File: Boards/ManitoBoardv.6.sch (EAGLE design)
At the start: 46 parts, among them U1 BLUETOOTH-RN41", U2 ATMEGA328P

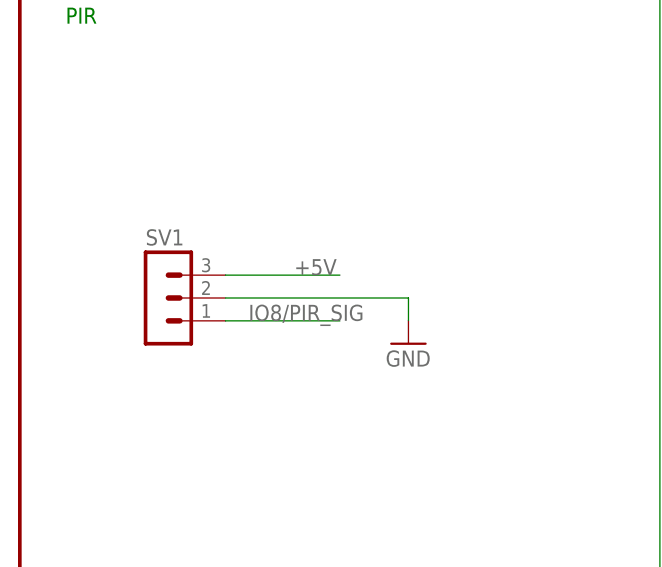
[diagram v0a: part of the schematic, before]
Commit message: Board with Layout
First complete layout now version .6
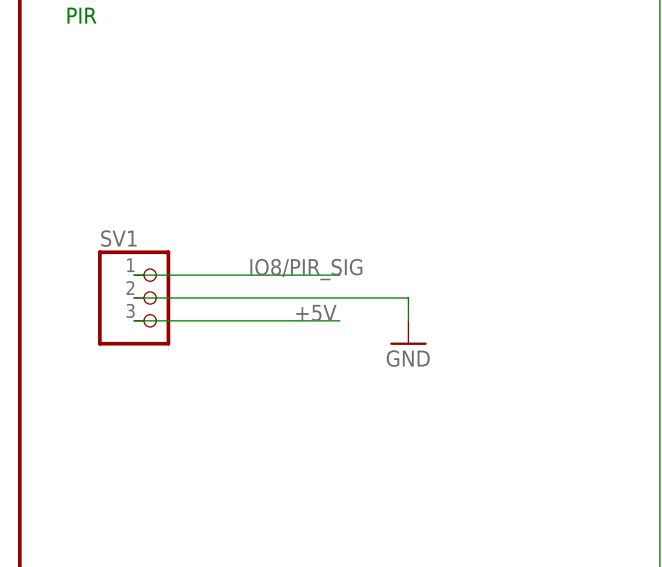
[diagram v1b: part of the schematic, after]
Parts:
- SV1: device con-lstb:MA03-1 -> adafruit:PINHD-1X3
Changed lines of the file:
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@@
 <part name="P+11" library="SparkFun" deviceset="VCC" device="" value="3.3V"/>
 <part name="P+4" library="supply1" deviceset="+5V" device=""/>
-<part name="SV1" library="con-lstb" deviceset="MA03-1" device=""/>
+<part name="SV1" library="adafruit" deviceset="PINHD-1X3" device=""/>
 <part name="GND14" library="supply1" deviceset="GND" device=""/>
 <part name="R17" library="SparkFun-Passives" deviceset="RESISTOR" device="PTH-1W" value="15"/>
@@
 <attribute name="VALUE" x="40.005" y="78.74" size="1.778" layer="96" rot="R180"/>
 </instance>
-<instance part="SV1" gate="G$1" x="15.24" y="363.22"/>
+<instance part="SV1" gate="A" x="15.24" y="363.22"/>
 <instance part="GND14" gate="1" x="43.18" y="358.14"/>
 <instance part="R17" gate="G$1" x="226.06" y="228.6" rot="R90"/>
@@
 </segment>
 <segment>
-<pinref part="SV1" gate="G$1" pin="2"/>
-<wire x1="22.86" y1="363.22" x2="43.18" y2="363.22" width="0.1524" layer="91"/>
+<pinref part="SV1" gate="A" pin="2"/>
+<wire x1="12.7" y1="363.22" x2="43.18" y2="363.22" width="0.1524" layer="91"/>
 <pinref part="GND14" gate="1" pin="GND"/>
 <wire x1="43.18" y1="363.22" x2="43.18" y2="360.68" width="0.1524" layer="91"/>
@@
 </segment>
 <segment>
-<pinref part="SV1" gate="G$1" pin="3"/>
-<wire x1="22.86" y1="365.76" x2="35.56" y2="365.76" width="0.1524" layer="91"/>
-<label x="30.48" y="365.76" size="1.778" layer="95"/>
+<pinref part="SV1" gate="A" pin="3"/>
+<wire x1="12.7" y1="360.68" x2="35.56" y2="360.68" width="0.1524" layer="91"/>
+<label x="30.48" y="360.68" size="1.778" layer="95"/>
 </segment>
 </net>
@@
 </segment>
 <segment>
-<pinref part="SV1" gate="G$1" pin="1"/>
-<wire x1="22.86" y1="360.68" x2="35.56" y2="360.68" width="0.1524" layer="91"/>
-<label x="25.4" y="360.68" size="1.778" layer="95"/>
-</segment>
-</net>
+<pinref part="SV1" gate="A" pin="1"/>
+<wire x1="12.7" y1="365.76" x2="35.56" y2="365.76" width="0.1524" layer="91"/>
+<label x="25.4" y="365.76" size="1.778" layer="95"/>
+</segment>
+</net>
